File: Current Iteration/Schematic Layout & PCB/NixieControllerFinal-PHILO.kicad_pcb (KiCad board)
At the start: 2 copper layers, 100 x 100 mm, 91 parts, among them J1 Conn_01x10_Pin, J2 USB_C_Receptacle_2.0, J3 Conn_01x10_Pin, J4 Conn_01x10_Pin, J5 Conn_01x10_Pin, J6 Conn_01x02, J7 Micro_SD_Card_Det1, J8 Conn_ARM_JTAG_SWD_10, J9 NixieIN, SW1 PEC11J-9215F-S0015, SW5 PEC16-2015F-N0024, SW6 PEC16-2015F-N0024, U1 HV5622PG, U10 NID1100, U11 TPS61040DBV, U13 STM32G0B1KEU6, U14 CM1224-04MR, U2 HV5622PG, U3 4504, U4 CM1224-04MR, U5 NCH6100HV, U6 CAP1206-x-SL, U7 NID1100, U8 MCP1700x-330xxTT, U9 MAX98357A

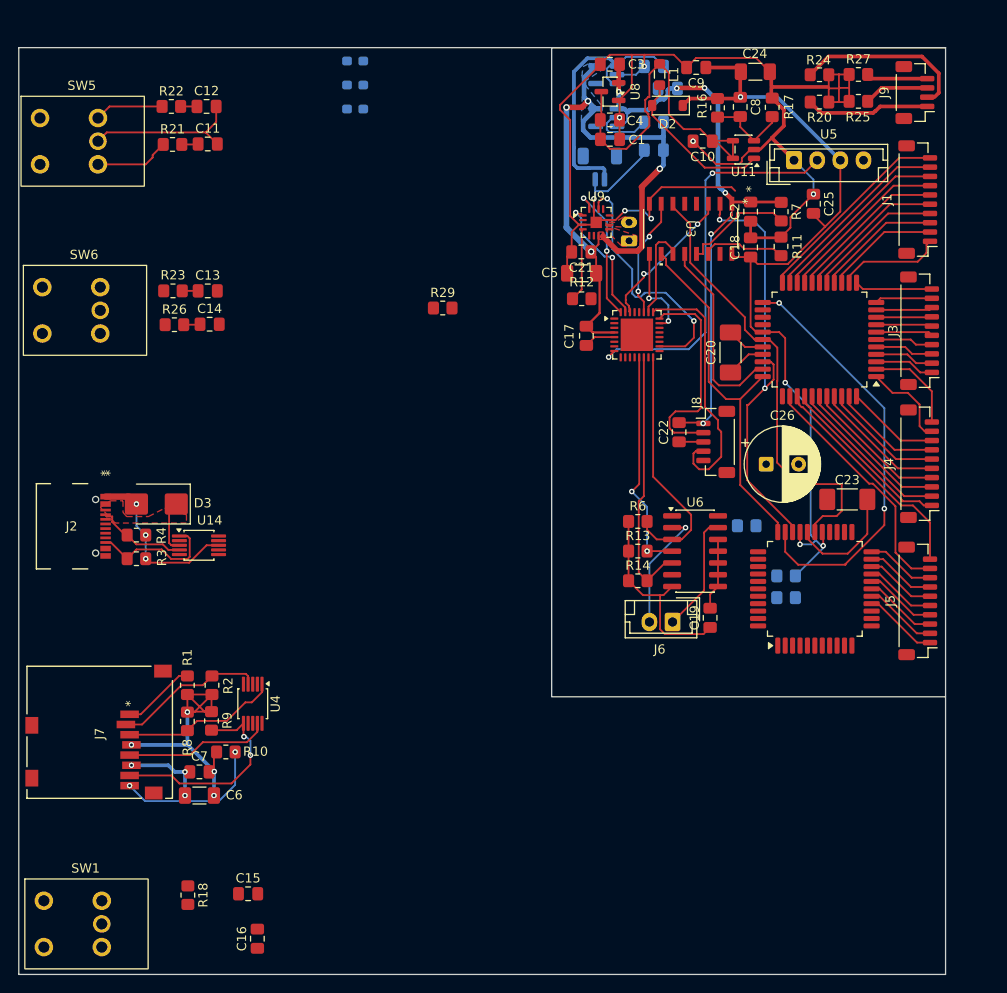
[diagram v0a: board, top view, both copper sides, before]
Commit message: readme update and schematic cleanup
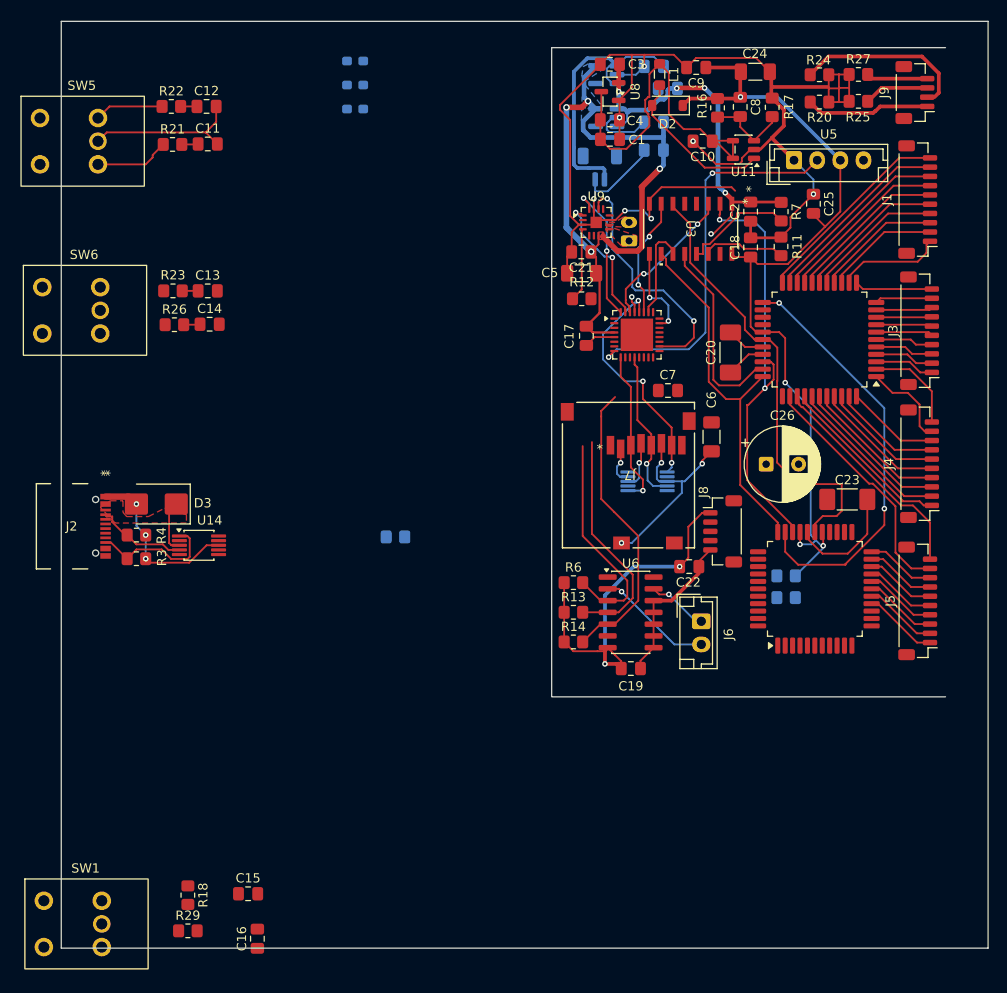
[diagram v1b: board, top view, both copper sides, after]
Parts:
- removed R1, R10, R2, R8, R9: 50k, Resistor_SMD:R_0805_2012Metric_Pad1.20x1.40mm_HandSolder
- C5: value 10uF -> 22uF
- U4: moved to B.Cu
- moved R29 72.6 mm to (127.7, 136.7)
- moved C6 67.5 mm to (184.2, 83.4), turned to -90 degrees
- moved C7 65.2 mm to (179.5, 78.4)
- moved J7 63.4 mm to (175.2, 87.5), turned to 180 degrees
- moved U4 48.9 mm to (177.3, 88.2), turned to 0 degrees
- moved R19 37.9 mm to (150.1, 94.2)
- moved C22 14.5 mm to (181.8, 97.4), turned to 0 degrees
- moved C19 10.2 mm to (175.5, 108.4), turned to 0 degrees
- moved J8 9.68 mm to (185.4, 93.6)
- moved U6 9.59 mm to (175.5, 102.3)
- moved R13 9.59 mm to (169.3, 102.3)
- moved R14 9.59 mm to (169.3, 105.5)
- moved R6 9.59 mm to (169.3, 99.1)
- moved J6 3.10 mm to (183.1, 103.3), turned to -90 degrees
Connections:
- J7 pad 1: Net-(J7-DAT2) -> unconnected-(J7-DAT2-Pad1)
- J7 pad 8: Net-(J7-DAT1) -> unconnected-(J7-DAT1-Pad8)
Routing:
- net +3.3V: track 121.5 -> 89.8 mm, vias 10 -> 8
- net /SWCLK: track 27.9 -> 0.00 mm
- net /SWDIO: track 23.3 -> 0.00 mm
- net GND: track 235.5 -> 255.2 mm
- net Net-(J7-DAT1): track 16.4 -> 0.00 mm, vias 2 -> 0
- net /SD_NSS: track 16.4 -> 4.16 mm, vias 0 -> 1
- net Net-(J7-DAT2): track 7.95 -> 0.00 mm
- net Net-(J6-Pin_1): track 12.8 -> 6.60 mm, vias 0 -> 1
- net /CAP_SCL: track 28.2 -> 32.1 mm
- net /SD_MISO: track 22.9 -> 25.9 mm, vias 2 -> 3
- net /CAP_INT: track 26.8 -> 24.1 mm
- net /ROT1A: track 0.00 -> 1.77 mm, vias 0 -> 1
- net /SD_SCK: track 15.7 -> 16.6 mm, vias 0 -> 1
- net /AU_LRCLK: track 27.4 -> 26.6 mm
- net Net-(J6-Pin_2): track 13.2 -> 12.6 mm
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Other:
- outline, holes or cut-outs redrawn

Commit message: Organization and CAD files
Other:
- board text added: "1"
- board text added: "2"
- board text added: "3"
- board text added: "4"
- board text added: "A"
- board text added: "A4"
- board text added: "ANGULAR:"
- board text added: "APPV'D"
- board text added: "B"
- board text added: "BREAK SHARP"
- board text added: "C"
- board text added: "CHK'D"
- board text added: "D"
- board text added: "DATE"
- board text added: "DEBURR AND"
- board text added: "DIMENSIONS ARE IN MILLIMETERS"
- board text added: "DO NOT SCALE DRAWING"
- board text added: "DRAWN"
- board text added: "DWG NO."
- board text added: "E"
- board text added: "EDGES"
- board text added: "F"
- board text added: "FINISH:"
- board text added: "For Instructional Use Only."
- board text added: "LINEAR:"
- board text added: "MATERIAL:"
- board text added: "MFG"
- board text added: "NAME"
- board text added: "NixieClock2"
- board text added: "Q.A"
- board text added: "REVISION"
- board text added: "SCALE:1:5"
- board text added: "SHEET 1 OF 1"
- board text added: "SIGNATURE"
- board text added: "SOLIDWORKS Educational Product."
- board text added: "SURFACE FINISH:"
- board text added: "TITLE:"
- board text added: "TOLERANCES:"
- board text added: "UNLESS OTHERWISE SPECIFIED:"
- board text added: "WEIGHT:"

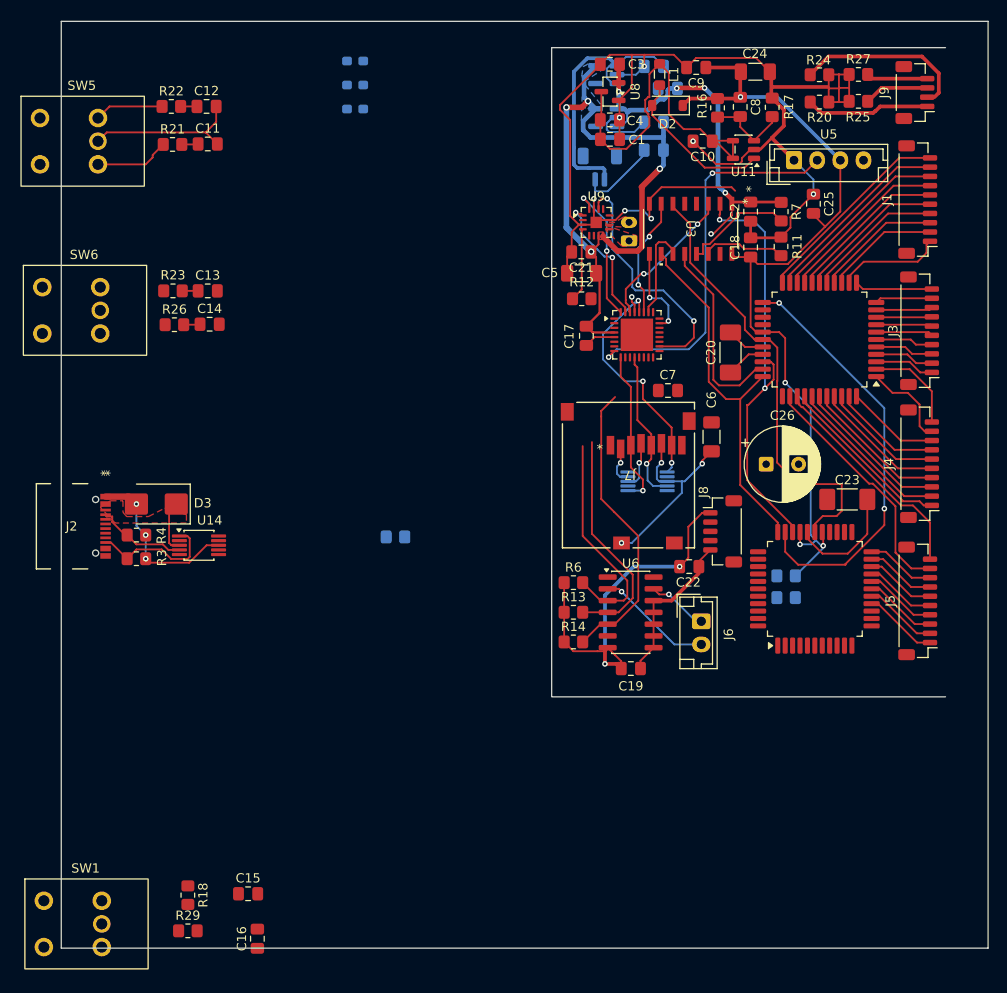
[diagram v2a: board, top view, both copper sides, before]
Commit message: repo refresh
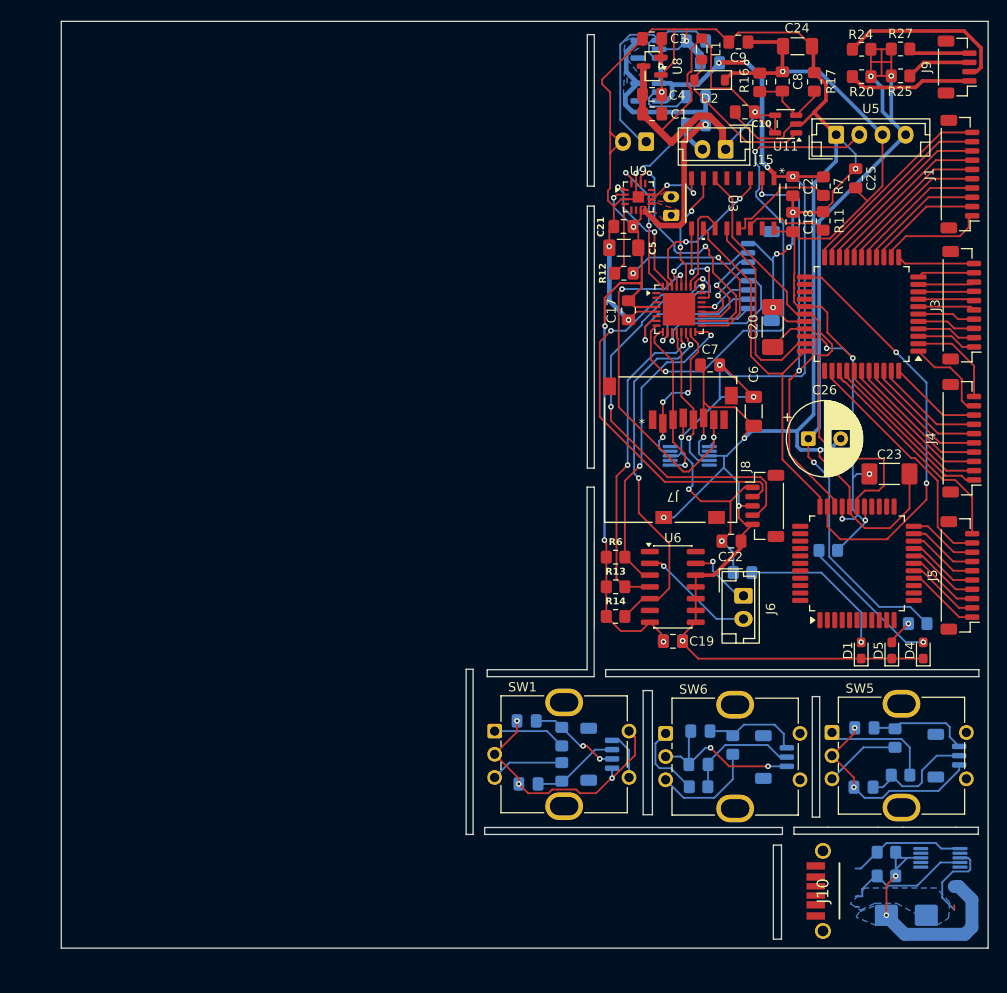
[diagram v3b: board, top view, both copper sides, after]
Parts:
- removed J2: USB_C_Receptacle_2.0, footprints:12402012E212A_AMP
- added C31: 1uF, Capacitor_SMD:C_0805_2012Metric_Pad1.18x1.45mm_HandSolder, B.Cu at (180.0, 105.4)
- added J10: 2480803-1, Connector_USB:24808031, F.Cu at (196.2, 132.4)
- added J11: Conn_01x04_Socket, Connector_JST:JST_SH_BM04B-SRSS-TB_1x04-1MP_P1.00mm_Vertical, B.Cu at (172.2, 117.7)
- added J12: Conn_01x03_Socket, Connector_JST:JST_SH_BM03B-SRSS-TB_1x03-1MP_P1.00mm_Vertical, B.Cu at (191.0, 118.0)
- added J13: Conn_01x03_Socket, Connector_JST:JST_SH_BM03B-SRSS-TB_1x03-1MP_P1.00mm_Vertical, B.Cu at (209.6, 117.8)
- added J15: Conn_01x02_Socket, Connector_JST:JST_EH_B2B-EH-A_1x02_P2.50mm_Vertical, F.Cu at (185.7, 52.4)
- added J16: Conn_01x08_Socket, Connector_JST:JST_SH_BM08B-SRSS-TB_1x08-1MP_P1.00mm_Vertical, B.Cu at (189.5, 66.0)
- BT1: footprint Connector_JST:JST_SH_BM02B-SRSS-TB_1x02-1MP_P1.00mm_Vertical -> Connector_JST:JST_EH_B2B-EH-A_1x02_P2.50mm_Vertical
- C11, C12, C13, C14, C15, C16, D3, R18, R21, R22, R23, R26, R29, R3, R4, U14: moved to B.Cu
- D1, D4, D5: moved to F.Cu
- SW1: value PEC11J-9215F-S0015 -> ~; footprint footprints:PEC09-2xxxF-Sxxxx -> Rotary_Encoder:RotaryEncoder_Bourns_Vertical_PEC12R-3x17F-Sxxxx
- SW5, SW6: value PEC16-2015F-N0024 -> ~; footprint footprints:PEC09-2xxxF-Sxxxx -> Rotary_Encoder:RotaryEncoder_Bourns_Vertical_PEC12R-3x17F-Sxxxx
- moved SW5 106.8 mm to (197.2, 115.3)
- moved R21 103.9 mm to (204.6, 119.9), turned to 180 degrees
- moved R22 103.6 mm to (204.0, 115.9), turned to -90 degrees
- moved C11 99.1 mm to (200.6, 121.2), turned to 180 degrees
- moved C12 97.6 mm to (200.7, 114.8), turned to 180 degrees
- moved D3 92.3 mm to (205.2, 135.0)
- moved R4 88.9 mm to (203.1, 130.8)
- moved R3 86.9 mm to (203.1, 128.2)
- moved U14 86.8 mm to (208.9, 128.8), turned to 180 degrees
- moved D4 86.5 mm to (207.1, 106.5), turned to 90 degrees
- moved D1 83.8 mm to (200.3, 106.5), turned to 90 degrees
- moved D5 82.3 mm to (203.7, 106.5), turned to 90 degrees
- moved SW6 81.5 mm to (179.2, 115.4)
- moved R23 77.8 mm to (186.5, 116.7), turned to -90 degrees
- moved R26 75.4 mm to (182.8, 121.2)
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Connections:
- net Net-(J6-Pin_1) renamed /CS_IN2
- net Net-(J6-Pin_2) renamed /CS_IN1
- net Net-(J9-Pin_1) renamed /HV_Vin4
- net Net-(J9-Pin_2) renamed /HV_Vin3
- net Net-(J9-Pin_3) renamed /HV_Vin2
- net Net-(J9-Pin_4) renamed /HV_Vin1
- C11 pad 1: /ROT2A -> Net-(J13-Pin_2)
- C11 pad 2: GND -> Net-(J13-Pin_3)
- C12 pad 1: /ROT2B -> Net-(J13-Pin_1)
- C12 pad 2: GND -> Net-(J13-Pin_3)
- C13 pad 1: /ROT3B -> Net-(J12-Pin_1)
- C13 pad 2: GND -> Net-(J12-Pin_3)
- C14 pad 1: /ROT3A -> Net-(J12-Pin_2)
- C14 pad 2: GND -> Net-(J12-Pin_3)
- C15 pad 1: /ROT1B -> Net-(J11-Pin_2)
- C15 pad 2: GND -> Net-(J11-Pin_4)
- C16 pad 1: /ROT1A -> Net-(J11-Pin_3)
- C16 pad 2: GND -> Net-(J11-Pin_4)
- C19 pad 1: +3.3V -> +V_CRIT
- D3 pad 1: +5V -> /5V_IN
- D3 pad 2: GND -> /GND1
- R13 pad 1: +3.3V -> +V_CRIT
- R14 pad 1: +3.3V -> +V_CRIT
- R18 pad 1: /ROT1B -> Net-(J11-Pin_2)
- R21 pad 2: /ROT2A -> Net-(J13-Pin_2)
- R22 pad 1: /ROT2B -> Net-(J13-Pin_1)
- R23 pad 1: /ROT3B -> Net-(J12-Pin_1)
- R26 pad 2: /ROT3A -> Net-(J12-Pin_2)
- R29 pad 2: /ROT1A -> Net-(J11-Pin_3)
- R3 pad 2: GND -> /GND1
- R4 pad 2: GND -> /GND1
- R6 pad 1: +3.3V -> +V_CRIT
- SW1 pad C: GND -> Net-(J11-Pin_4)
- SW1 pad S1: GND -> Net-(J11-Pin_4)
- SW1 pad S2: /SELECT_RET -> Net-(J11-Pin_1)
- SW5 pad C: GND -> Net-(J13-Pin_3)
- SW6 pad C: GND -> Net-(J12-Pin_3)
- U13 pad 11: unconnected-(U13-PA4-Pad11) -> /ROT2B
- U14 pad 3: +5V -> /5V_IN
- U14 pad 8: GND -> /GND1
- U6 pad 7: +3.3V -> +V_CRIT
- U9 pad 2: unconnected-(U9-GAIN_SLOT-Pad2) -> +V_CRIT
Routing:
- net +170V: track 0.00 -> 92.4 mm, vias 0 -> 3
- net GND: track 255.2 -> 321.2 mm, vias 13 -> 18
- net /SWCLK: track 0.00 -> 47.8 mm, vias 0 -> 2
- net /SWDIO: track 0.00 -> 45.1 mm, vias 0 -> 2
- net +V_CRIT: track 70.9 -> 105.0 mm, vias 4 -> 6
- net /GND1: track 0.00 -> 28.6 mm, vias 0 -> 2
- net Net-(J11-Pin_4): track 0.00 -> 27.8 mm, vias 0 -> 3
- net +3.3V: track 89.8 -> 114.4 mm, vias 8 -> 10
- net Net-(J13-Pin_3): track 0.00 -> 22.0 mm, vias 0 -> 2
- net /AU_~{SD}: track 0.00 -> 21.6 mm, vias 0 -> 2
- net Net-(J12-Pin_3): track 0.00 -> 18.7 mm, vias 0 -> 2
- net Net-(D1-A): track 0.00 -> 16.8 mm, vias 0 -> 1
- net Net-(D4-A): track 0.00 -> 15.7 mm, vias 0 -> 1
- net /ROT3B: track 1.71 -> 16.6 mm, vias 0 -> 1
- net /ROT2B: track 1.76 -> 16.7 mm, vias 0 -> 1
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- added copper zone on B.Cu, net /5V_IN
- added copper zone on B.Cu, net /GND1
- removed copper zone on F.Cu, net +5V
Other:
- outline, holes or cut-outs redrawn
